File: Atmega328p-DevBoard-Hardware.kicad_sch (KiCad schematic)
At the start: 28 parts, among them J1 Barrel_Jack, J2 DBG/PROG, J3 MTR1-CON, J4 MTR2-CON, SW1 SW_SPST, U1 L7805, U2 ATmega328P-A, U3 L293D, Y1 LFXTAL003237-Crystal-16MHz

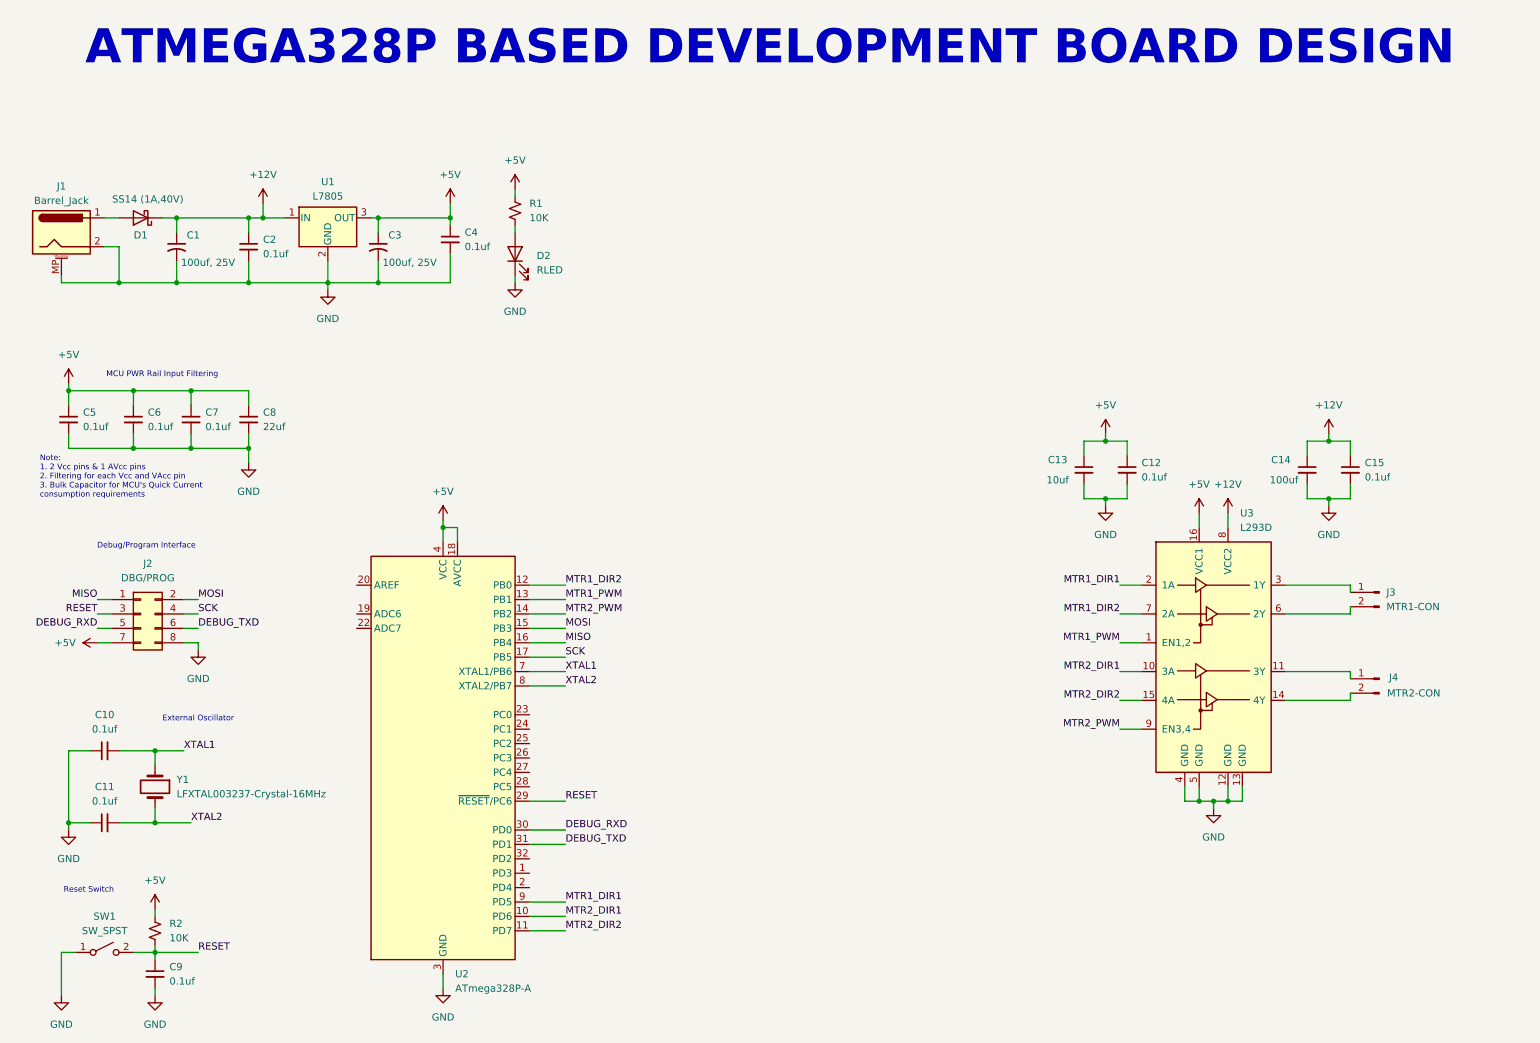
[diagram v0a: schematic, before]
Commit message: completed ssd section
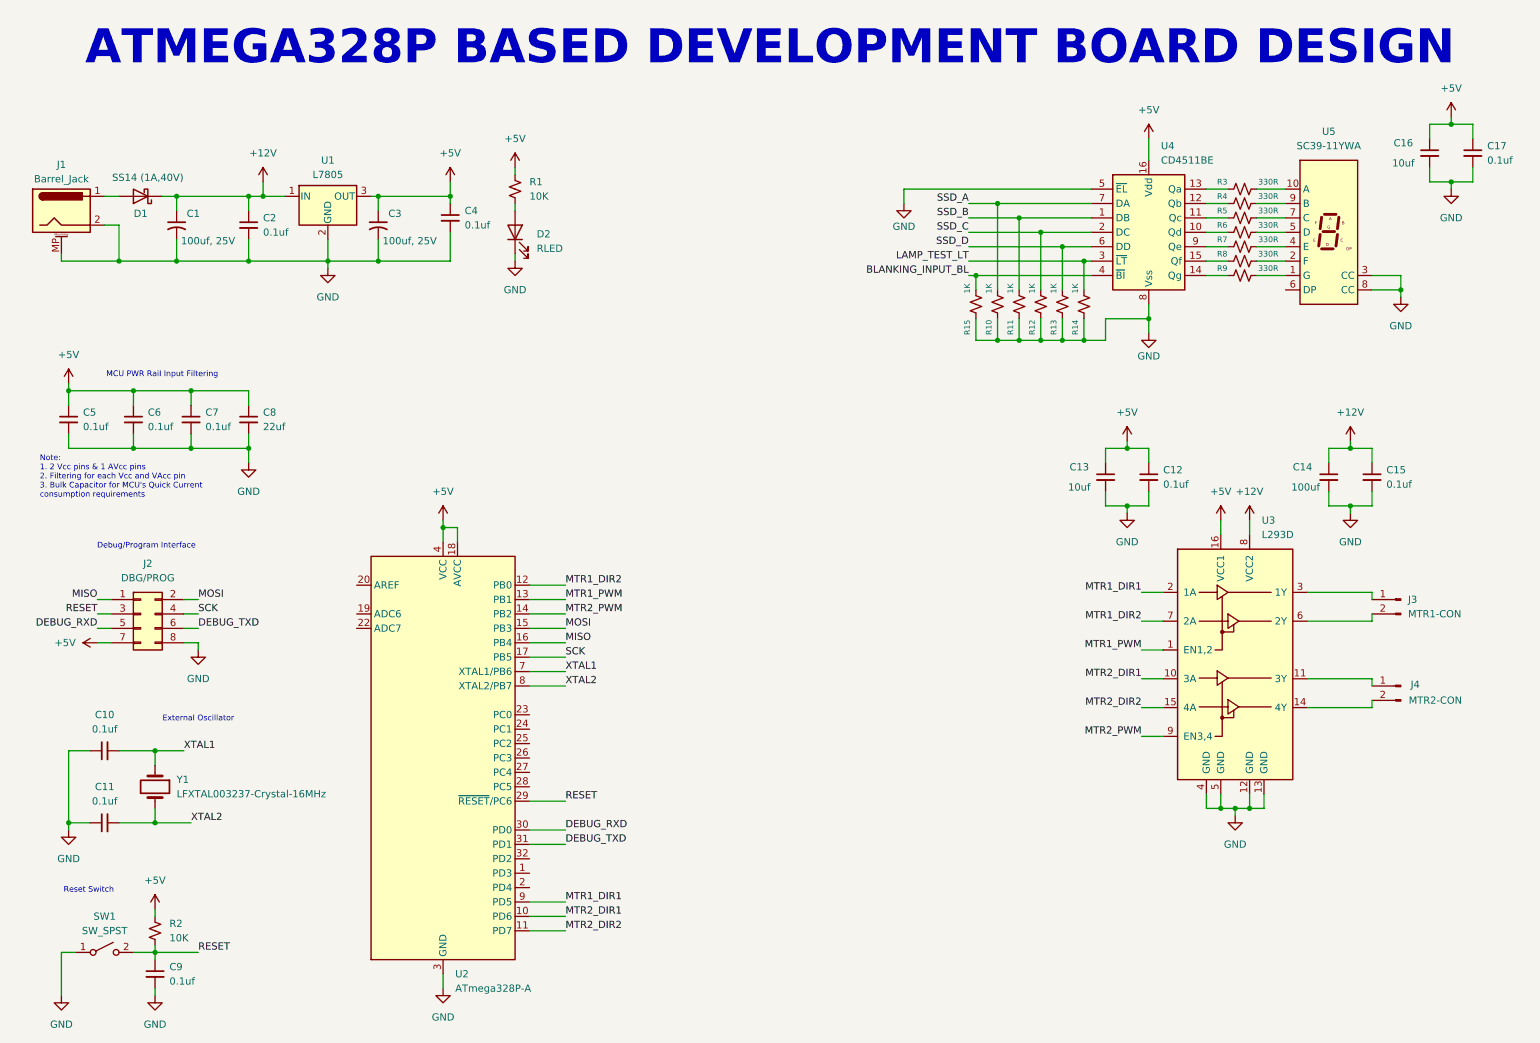
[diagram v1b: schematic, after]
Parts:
- added C16: 10uf, Capacitor_SMD:C_0805_2012Metric_Pad1.18x1.45mm_HandSolder, symbol Device:C_Small
- added C17: 0.1uf, Capacitor_SMD:C_0805_2012Metric_Pad1.18x1.45mm_HandSolder, symbol Device:C_Small
- added R10, R11, R12, R13, R14, R15: 1K, Resistor_SMD:R_0805_2012Metric_Pad1.20x1.40mm_HandSolder, symbol Device:R_Small_US
- added R3, R4, R5, R6, R7, R8, R9: 330R, Resistor_SMD:R_0805_2012Metric_Pad1.20x1.40mm_HandSolder, symbol Device:R_Small_US
- added U4: CD4511BE, Package_DIP:DIP-16_W7.62mm_LongPads, symbol 4xxx_IEEE:4511
- added U5: SC39-11YWA, Display_7Segment:Sx39-1xxxxx, symbol Display_Character:SC39-11YWA
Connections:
- net +5V: now also C16.1, C17.1, U4.16 (Vdd)
- net GND: now also C16.2, C17.2, R10.1, R11.1, R12.1, R13.1, R14.1, R15.1, U4.5 (~{EL}), U4.8 (Vss), U5.3 (CC), U5.8 (CC)
- new net: R5.1, U4.11 (Qc)
- new net: R5.2, U5.7 (C)
- new net: R7.1, U4.9 (Qe)
- new net: R7.2, U5.4 (E)
- new net: R3.1, U4.13 (Qa)
- new net: R3.2, U5.10 (A)
- new net: R6.1, U4.10 (Qd)
- new net: R6.2, U5.5 (D)
- new net: R8.1, U4.15 (Qf)
- new net: R8.2, U5.2 (F)
- new net: R4.1, U4.12 (Qb)
- new net: R4.2, U5.9 (B)
- new net: R9.1, U4.14 (Qg)
- new net: R9.2, U5.1 (G)
- new net BLANKING_INPUT_BL: R15.2, U4.4 (~{BI})
- new net LAMP_TEST_LT: R14.2, U4.3 (~{LT})
- new net SSD_A: R10.2, U4.7 (DA)
- new net SSD_B: R11.2, U4.1 (DB)
- new net SSD_C: R12.2, U4.2 (DC)
- new net SSD_D: R13.2, U4.6 (DD)
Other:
- moved on the sheet: C1, C12, C13, C14, C15, C2, C3, C4, D1, D2, J1, J3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
